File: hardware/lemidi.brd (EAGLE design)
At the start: 100 x 100 mm, 66 parts, among them Q1 IRLML6246, Q2 IRLML6246, Q3 IRLML6246, Q4 IRLML6246, U1 SPX5205 3v3, X1 MOLEX_2HORIZONTAL, X3 MOLEX_6HORIZONTAL, Y1 32768Hz CFPX-217 12.5pF, Y2 12MHz 0.25%, Y3 8MHz

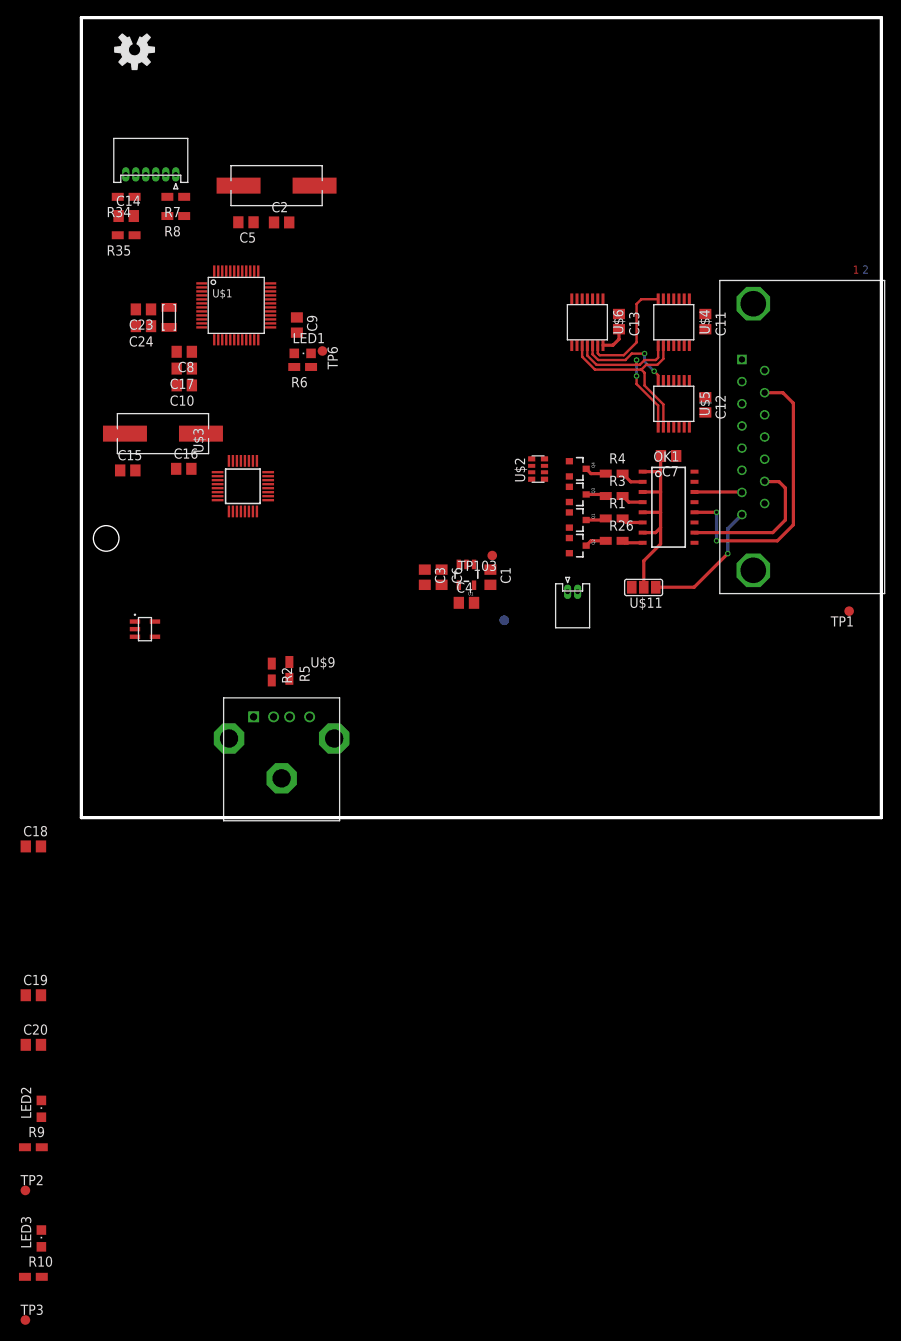
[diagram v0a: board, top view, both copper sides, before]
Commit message: happy new year
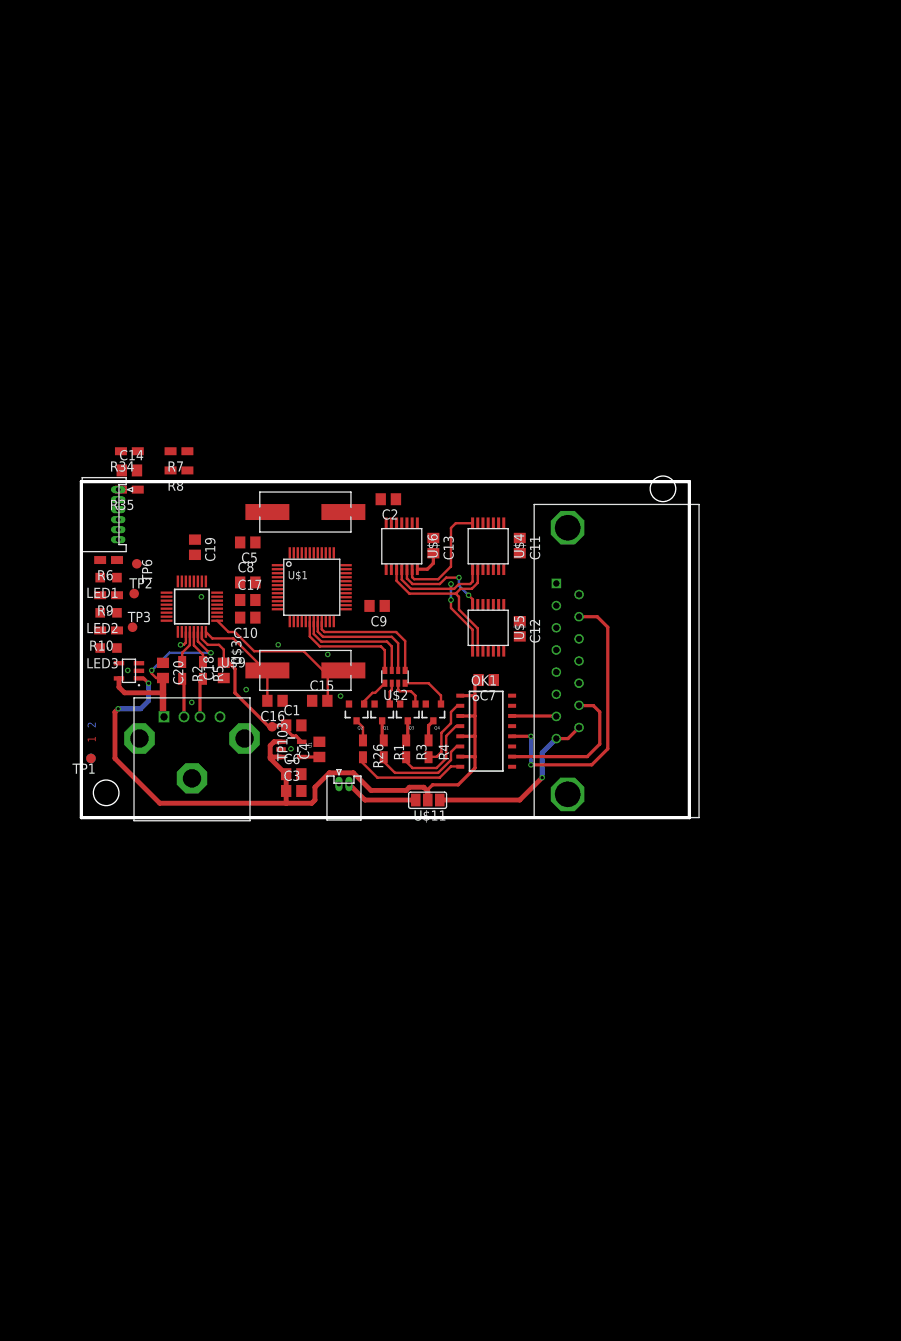
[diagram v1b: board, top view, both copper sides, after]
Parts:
- removed C23, C24: 22pF, rcl:C0805
- removed Y1: 32768Hz CFPX-217 12.5pF, Simplex-FreqCtrl:CRYSTAL-SMD-3.2X1.5
- moved U$7 112.4 mm to (71.8, 4.35), flipped to the bottom, turned to 90 degrees
- moved TP1 96.5 mm to (1.20, 7.40)
- moved TP3 87.6 mm to (6.40, 23.8)
- moved R10 81.3 mm to (3.40, 23.4), turned to 180 degrees
- moved TP2 75.8 mm to (6.60, 28.0)
- moved LED3 74.3 mm to (3.40, 21.2), turned to 90 degrees
- moved R9 69.6 mm to (3.40, 27.8), turned to 180 degrees
- moved LED2 62.6 mm to (3.40, 25.6), turned to 90 degrees
- moved C19 59.5 mm to (14.2, 33.8), turned to 270 degrees
- moved TP101 54.5 mm to (1.20, 7.40)
- moved C20 49.5 mm to (10.2, 18.4), turned to 270 degrees
- moved R4 41.5 mm to (43.4, 8.60), turned to 270 degrees
- moved Y3 41.0 mm to (28.0, 38.2)
- moved R3 40.9 mm to (40.6, 8.60), turned to 270 degrees
- moved R26 40.8 mm to (35.2, 8.60), turned to 270 degrees
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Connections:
- net N$1 renamed 12MHZ_XO
- net N$3 renamed 12MHX_XI
- removed net N$25: C24.1, U$1.9, Y1.P$1
- removed net N$26: C23.1, U$1.8, Y1.P$2
- removed net VIN: C3.1, C6.1, U1.1, U1.3
- new net N$1: LED1.A, R6.2
- new net N$20: U$1.20, U$2.2
- new net N$21: U$1.21, U$2.1
- new net N$3: U$1.18, U$2.4
- net +5V: now also C3.1, C6.1, U1.1, U1.3
- net B1_EN: now also U$2.8
- net B2_EN: now also U$2.7
- net B3_EN: now also U$2.6
- net B4_EN: now also U$2.5
- net GND: now also LED1.C, LED2.C, LED3.C; no longer C23.2, C24.2, R10.2, R6.2, R9.2
- net N$11: now also LED3.A, R10.2; no longer LED3.C, R10.1
- net N$4: now also LED2.A, R9.2; no longer LED2.C, R9.1
- net N$8: now also U$1.19, U$2.3; no longer LED1.C, R6.1
- net STATUS: now also R6.1; no longer LED1.A
- net USB_GPX: now also U$1.15
- net USB_INT: now also U$1.14
- net USB_ST1: now also R9.1; no longer LED2.A
- net USB_ST2: now also R10.1; no longer LED3.A
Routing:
- net +5V: track 30.1 -> 102.3 mm, vias 0 -> 2
- net VBUS: track 0.00 -> 25.7 mm, vias 0 -> 2
- net 12MHZ_XO: track 0.00 -> 22.2 mm
- net +3V3: track 0.00 -> 21.8 mm
- net N$21: track 0.00 -> 15.7 mm
- net N$20: track 0.00 -> 15.3 mm
- net N$8: track 0.00 -> 14.9 mm
- net N$3: track 0.00 -> 14.5 mm
- net 12MHX_XI: track 0.00 -> 13.5 mm
- net N$9: track 2.61 -> 14.4 mm
- net N$7: track 2.72 -> 12.6 mm
- net 5V_EXT: track 0.00 -> 9.18 mm
- net N$13: track 2.82 -> 11.5 mm
- net 5V_PC: track 16.4 -> 23.0 mm
- net B1_EN: track 0.00 -> 6.17 mm
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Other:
- board size 100 x 100 mm -> 76 x 42 mm
- board text added: "github.com/rodan/lemidi"
- board text removed: "+3V3"
- board text removed: "github.com/rodan/retrojoy"
- board text removed: "status"
- board text removed: "tp1"
- board text removed: "tp2"
- board text removed: "tp3"
- board text removed: "tp4"
- board text removed: "tp5"
- board text removed: "tp6"
